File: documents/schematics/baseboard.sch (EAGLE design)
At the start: 37 parts, among them IC1 MAX 604, IC2 AD780N, J1 350792-1, Q1 20 MHz, Q2 BS170, Q3 BS170, Q4 5 MHz, T1 2N3904

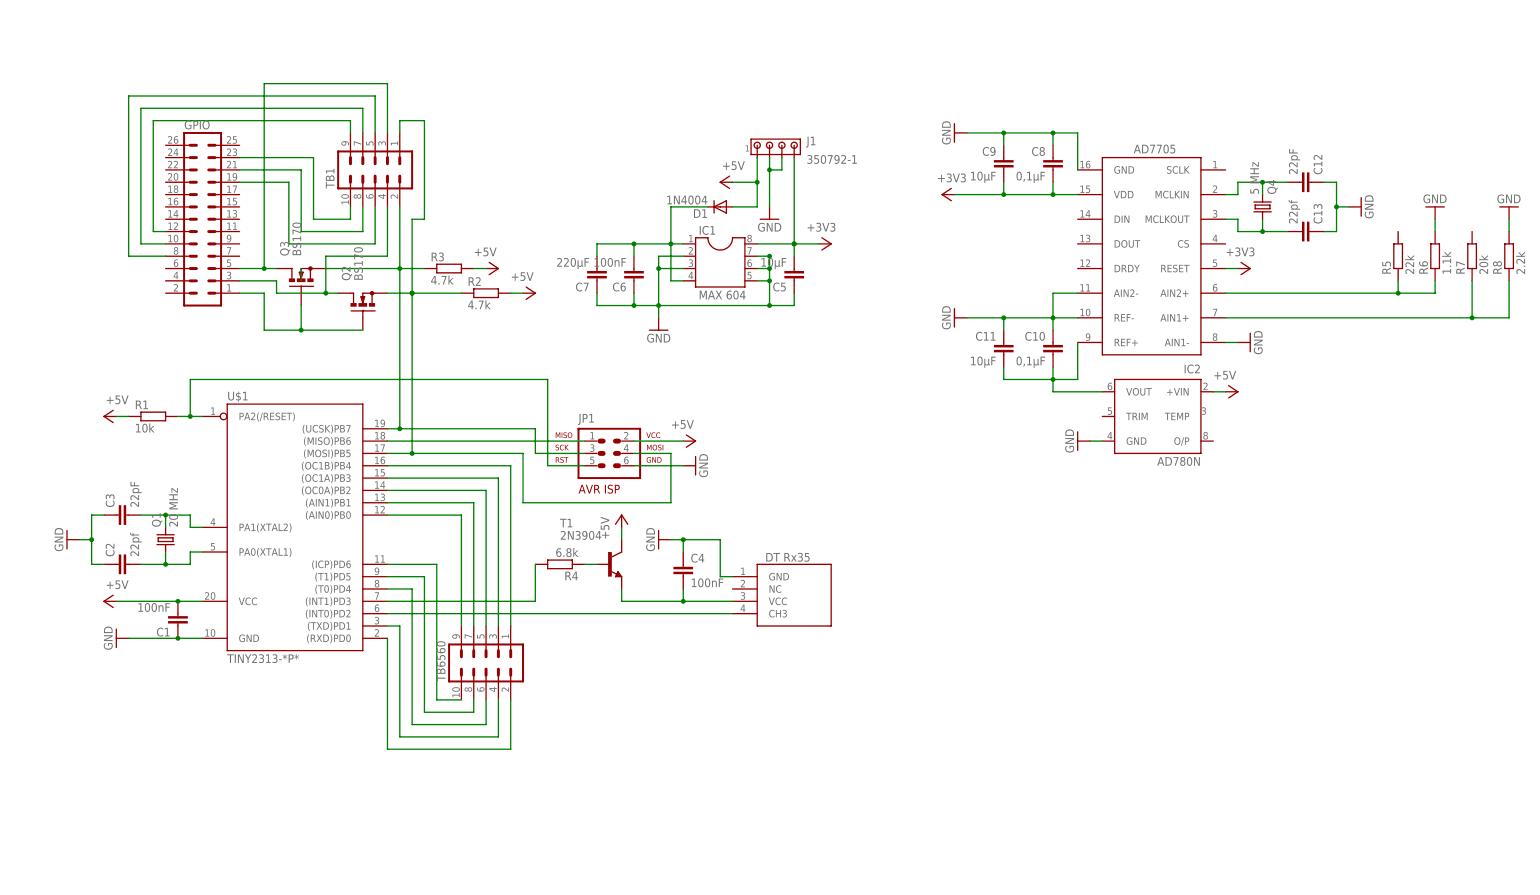
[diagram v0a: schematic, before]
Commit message: Baseboard alpha
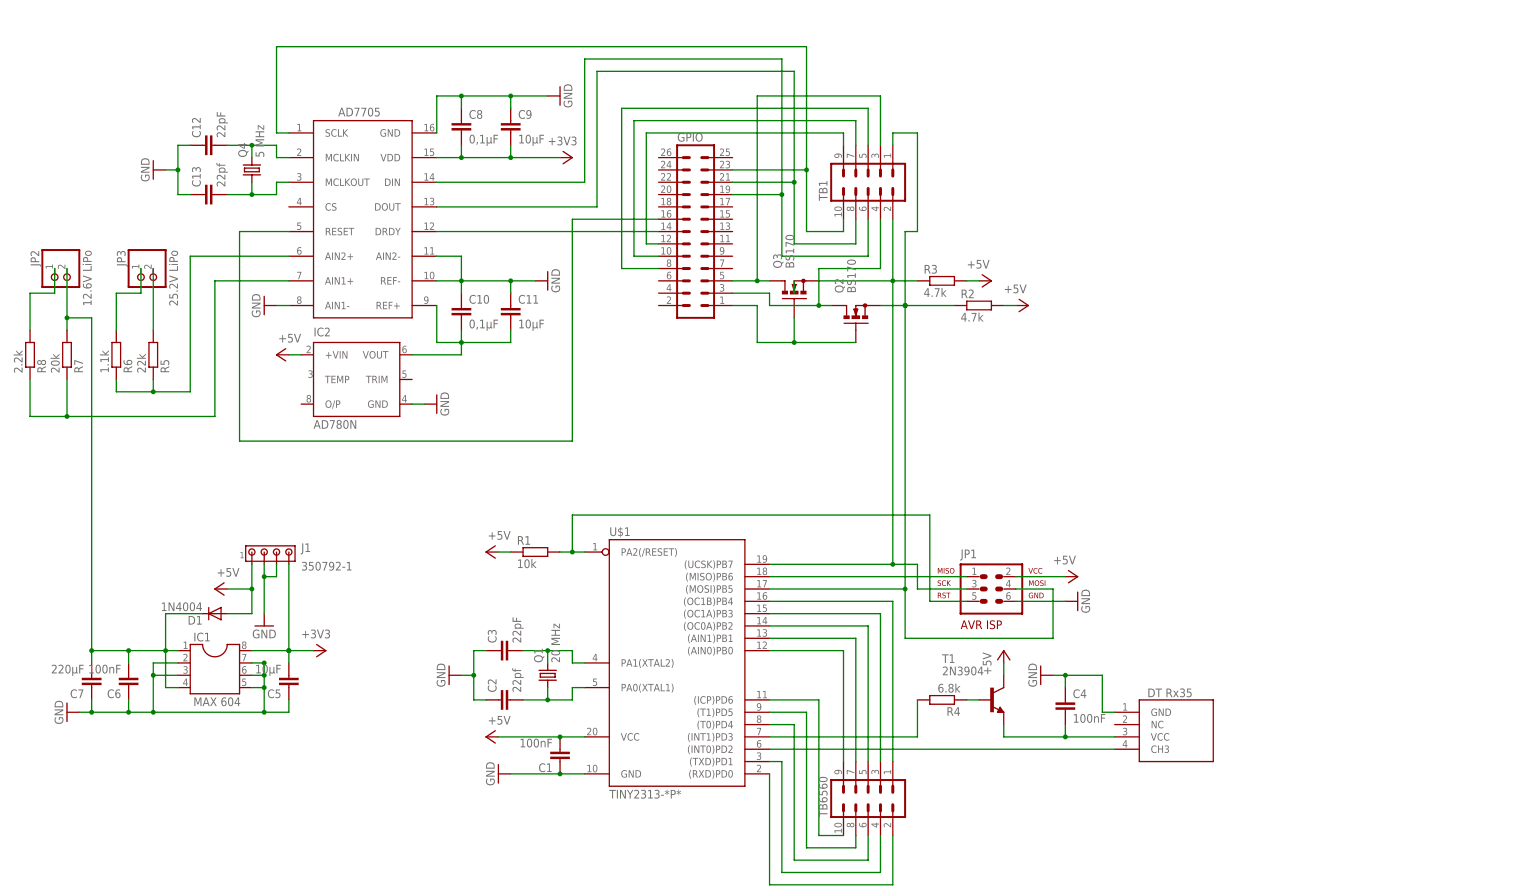
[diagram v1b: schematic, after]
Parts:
- added JP2: 12.6V LiPo, pinhead:PINHD-1X2
- added JP3: 25.2V LiPo, pinhead:PINHD-1X2
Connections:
- new net N$33: JP3.1, R6.2
- new net N$34: JP2.1, R8.2
- new net N$39: JP3.2, R5.2
- new net N$42: GPIO.14, U$3.DRDY
- new net N$43: GPIO.16, U$3.RESET
- net +3V3: no longer U$3.RESET
- net GND: no longer R6.2, R8.2
- net N$27: now also U$3.SCLK
- net N$29: now also U$3.DOUT
- net N$30: now also U$3.DIN
- net N$32: now also JP2.2, R7.2
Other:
- moved on the sheet: C1, C10, C11, C12, C13, C2, C3, C4, C5, C6, C7, C8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

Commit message: Baseboard Bugfix
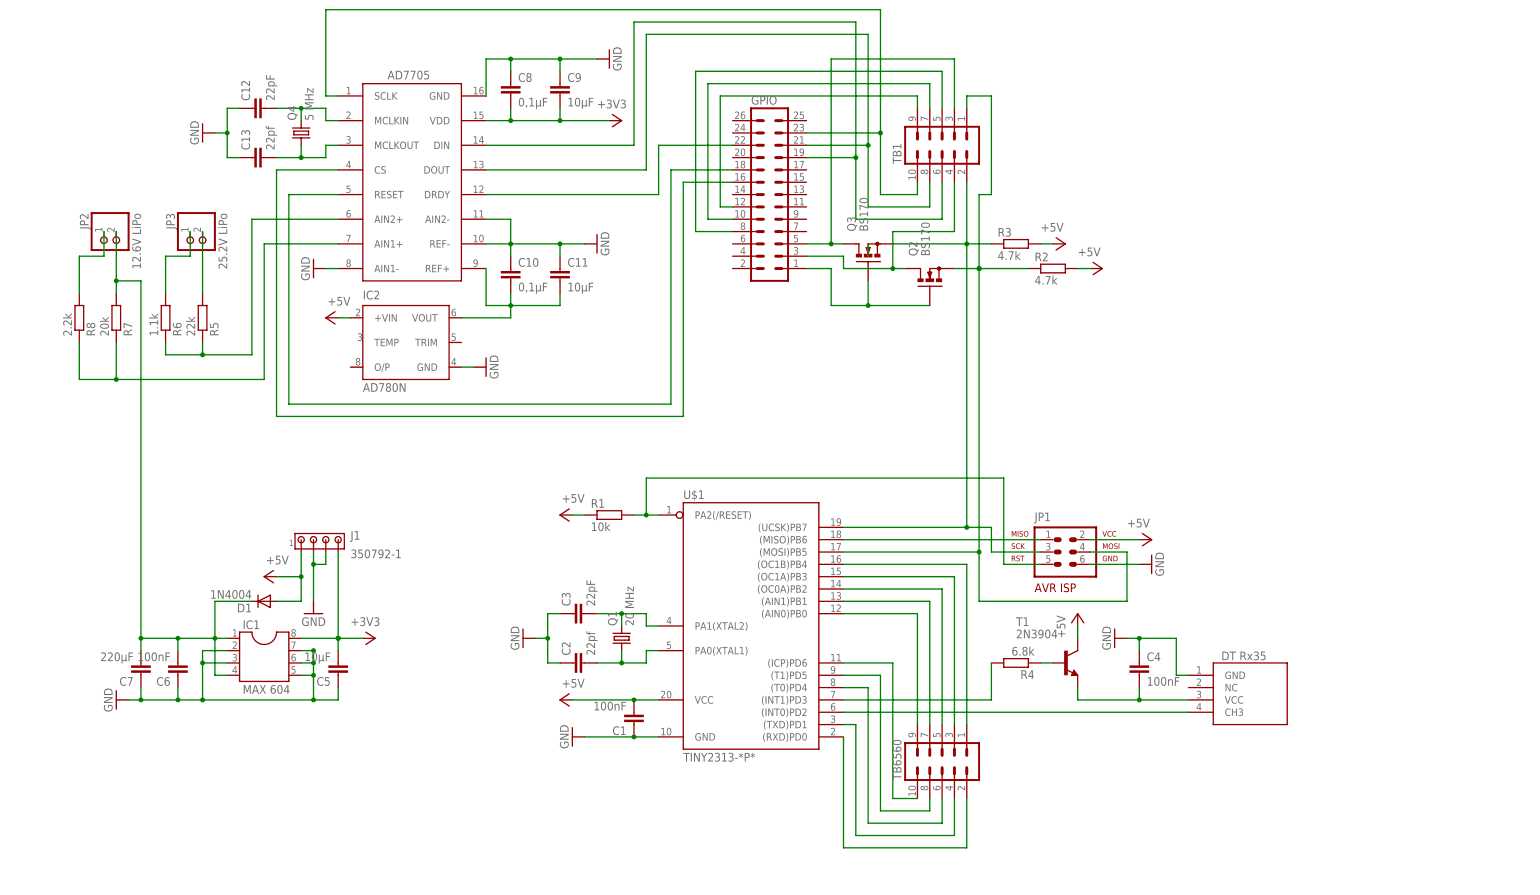
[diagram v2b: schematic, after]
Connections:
- removed net N$42: GPIO.14, U$3.DRDY
- new net N$40: GPIO.22, U$3.DRDY
- new net N$41: GPIO.16, U$3.CS
- net N$43: now also GPIO.18; no longer GPIO.16
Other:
- moved on the sheet: C1, C10, C11, C12, C13, C2, C3, C4, C5, C6, C7, C8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
